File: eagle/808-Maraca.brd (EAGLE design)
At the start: 100 x 80 mm, 45 parts, among them IC1 TL071P, Q1 2N3904, Q2 2N3906, Q3 2N3906, Q4 2N3904, Q59 2N3904, Q60 2N3906

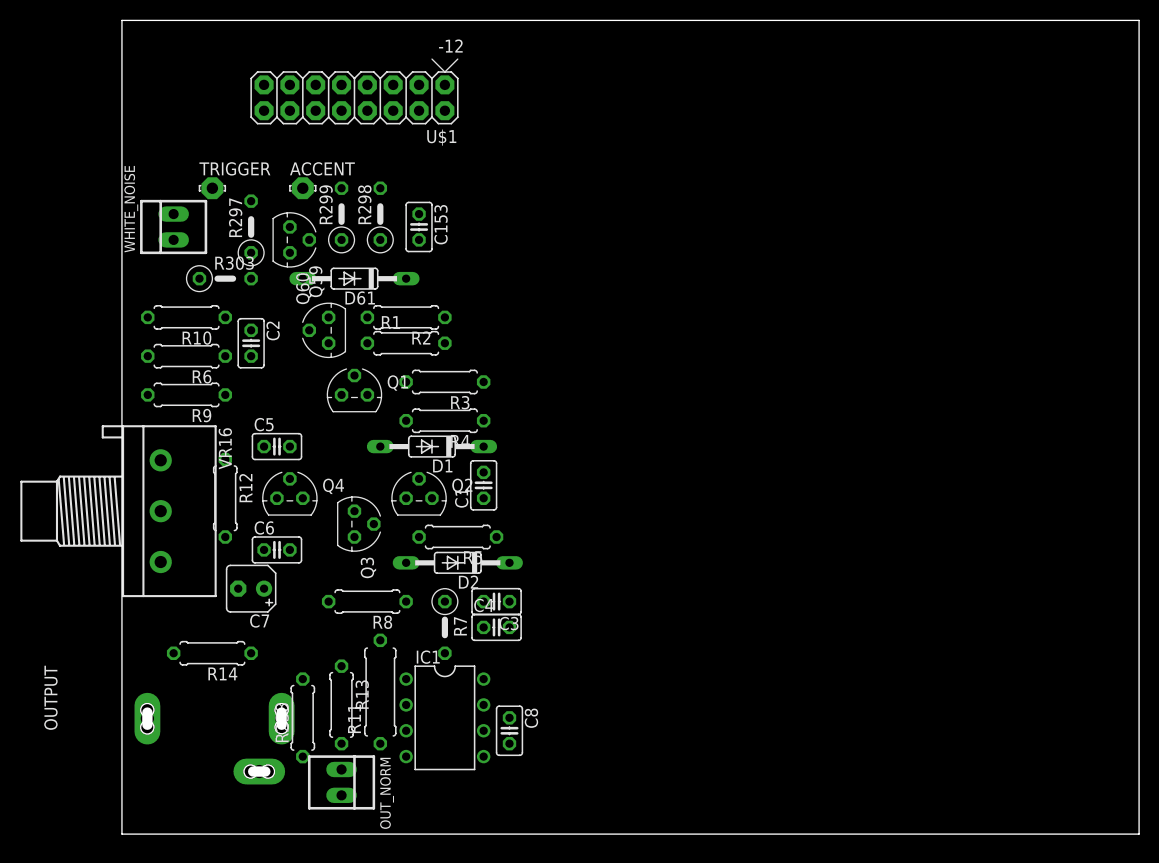
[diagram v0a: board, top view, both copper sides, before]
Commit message: tweaks
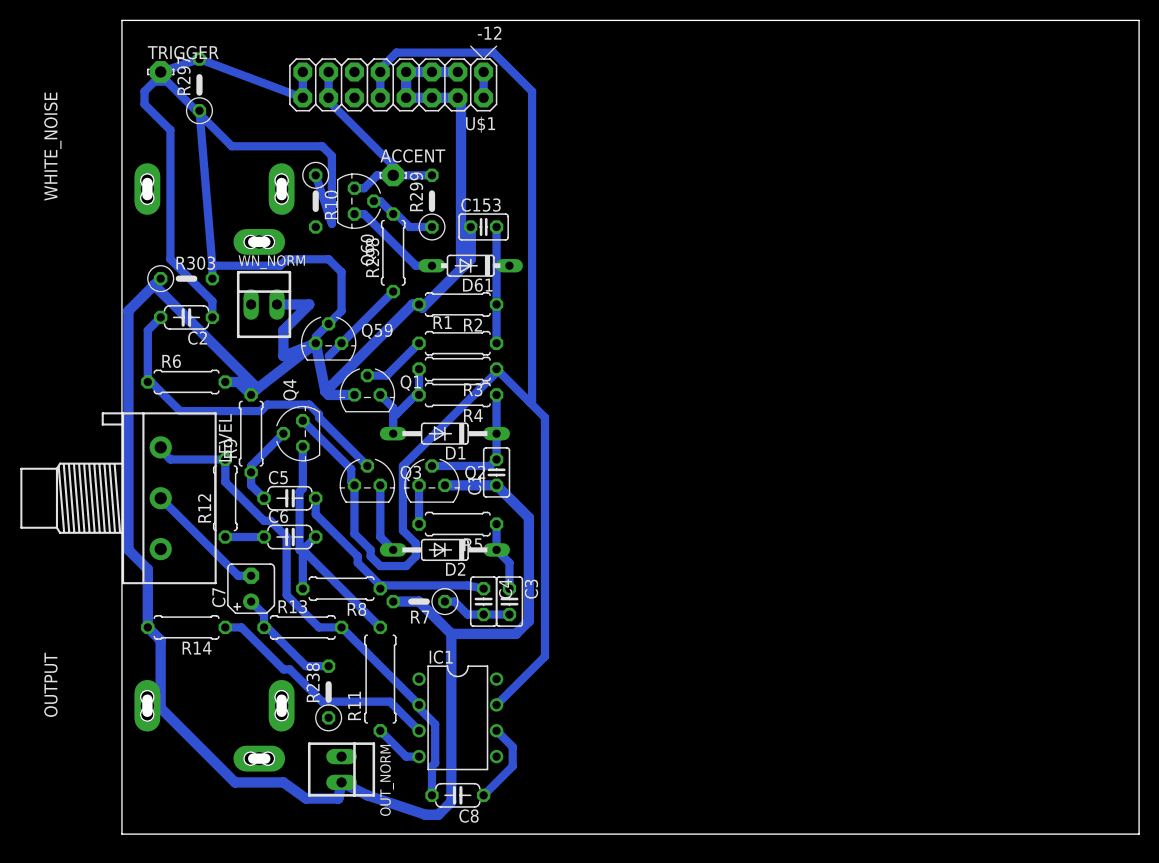
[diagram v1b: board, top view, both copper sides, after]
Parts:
- removed VR16: 100KA, pot:3RP/1610N
- added LEVEL: 100KA, pot:3RP/1610N
- added WN_NORM: 22-23-2021, con-molex:22-23-2021
- C2, C5, C6, C8: device TR808clone:C025-025X050 -> TR808clone:C050-024X044
- D61: value 1N4148DO35-10 -> 1N4148DO35-7; device TR808clone:DO35-10 -> TR808clone:DO35-7
- R10, R238: device TR808clone:0207/7 -> TR808clone:0207/5V
- R298: device TR808clone:0207/5V -> TR808clone:0207/7
- WHITE_NOISE: value 22-23-2021 -> AUDIO-JACK; device con-molex:22-23-2021 -> erthenvar:ERTHENVAR-JACK-90DEG
- moved R10 17.1 mm to (19.1, 62.2), turned to 270 degrees
- moved R297 14.9 mm to (7.62, 73.7)
- moved TRIGGER 12.5 mm to (3.81, 74.9)
- moved D61 11.5 mm to (34.3, 55.9)
- moved ACCENT 8.98 mm to (26.7, 64.8)
- moved R299 8.98 mm to (30.5, 62.2)
- moved R13 8.52 mm to (17.8, 20.3), turned to 0 degrees
- moved C8 8.13 mm to (33.0, 3.81), turned to 180 degrees
- moved R9 7.41 mm to (12.7, 39.4), turned to 90 degrees
- moved Q60 7.41 mm to (22.9, 62.2)
- moved C2 6.84 mm to (6.35, 50.8), turned to 180 degrees
- moved Q4 6.48 mm to (17.8, 39.4), turned to 90 degrees
- moved C153 6.35 mm to (35.6, 59.7), turned to 0 degrees
- moved R2 5.24 mm to (33.0, 52.1)
- moved WHITE_NOISE 5.24 mm to (0.00, 58.4)
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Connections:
- new net N$21: WHITE_NOISE.P$2, WN_NORM.1
- net GND: now also WHITE_NOISE.P$1, WN_NORM.2; no longer WHITE_NOISE.2
- net N$17: now also LEVEL.1; no longer VR16.1
- net N$19: now also LEVEL.2; no longer VR16.2
- net N$6: now also WHITE_NOISE.P$3; no longer WHITE_NOISE.1
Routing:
- net GND: track 0.00 -> 229.6 mm
- net +12V: track 0.00 -> 131.8 mm
- net N$14: track 0.00 -> 58.5 mm
- net N$17: track 0.00 -> 50.4 mm
- net N$318: track 0.00 -> 37.5 mm
- net N$11: track 0.00 -> 32.6 mm
- net N$16: track 0.00 -> 26.9 mm
- net N$22: track 0.00 -> 23.3 mm
- net N$13: track 0.00 -> 21.8 mm
- net TRIG: track 0.00 -> 21.6 mm
- net N$8: track 0.00 -> 19.2 mm
- net N$20: track 0.00 -> 17.4 mm
- net N$4: track 0.00 -> 13.0 mm
- net N$324: track 0.00 -> 12.7 mm
- net N$19: track 0.00 -> 12.0 mm
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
